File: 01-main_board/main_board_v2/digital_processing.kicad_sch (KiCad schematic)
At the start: 34 parts, among them IC9 LSF0108PWR, T1 749013011

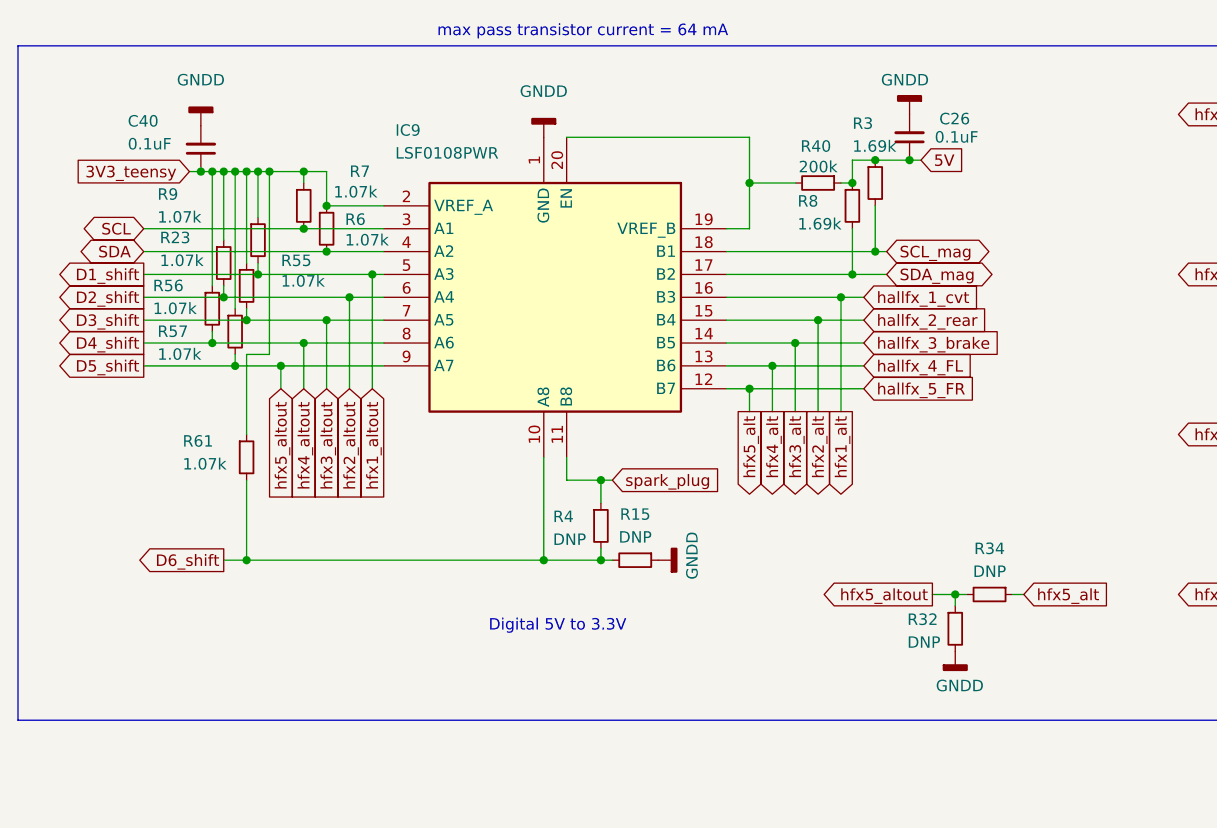
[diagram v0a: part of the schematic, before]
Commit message: made progress on layout
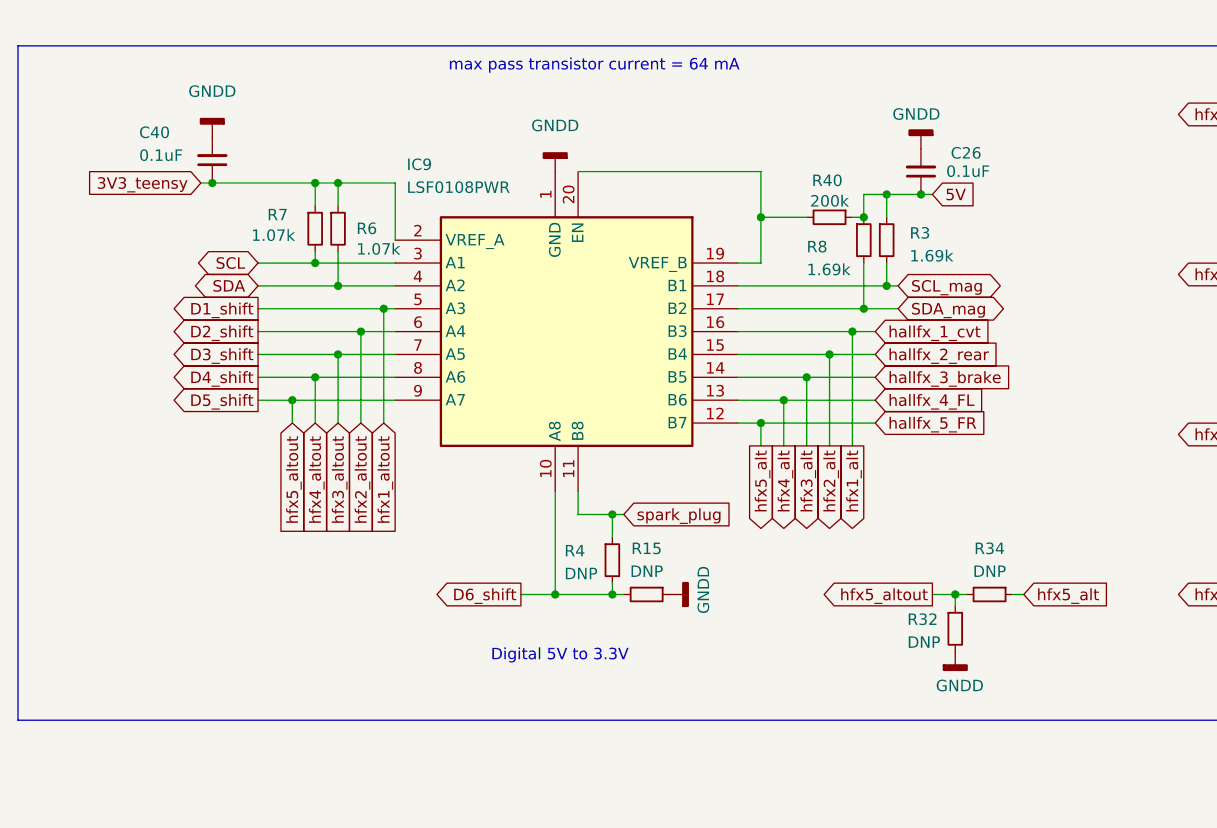
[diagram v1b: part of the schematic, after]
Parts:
- removed R23, R55, R56, R57, R61, R9: 1.07k, Resistor_SMD:R_0402_1005Metric, symbol Device:R_Small
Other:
- moved on the sheet: C26, C40, IC9, R15, R3, R4, R40, R6, R7, R8
